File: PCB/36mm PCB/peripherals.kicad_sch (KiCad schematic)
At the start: 21 parts, among them IC2 BMM350, IC6 AS5510-DWLM, J1 Conn_01x04_Pin, U1 BMP581

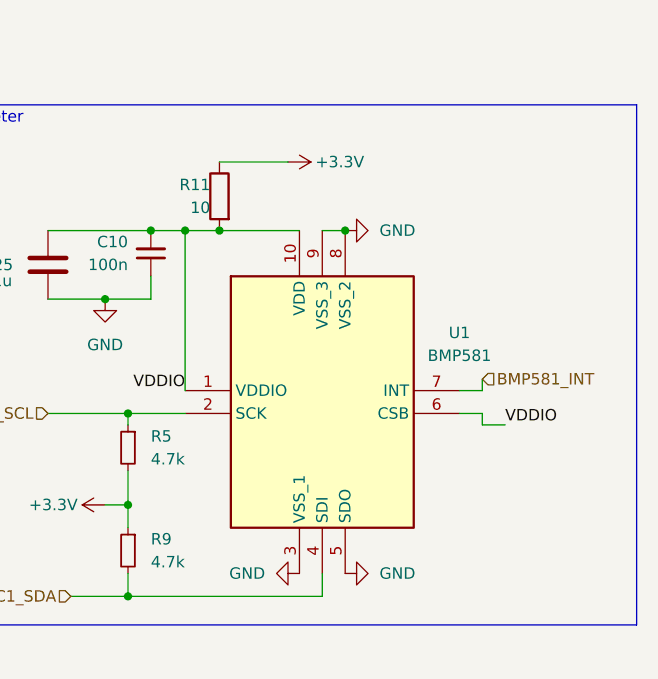
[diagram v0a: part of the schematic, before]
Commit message: Modifs Mathieu
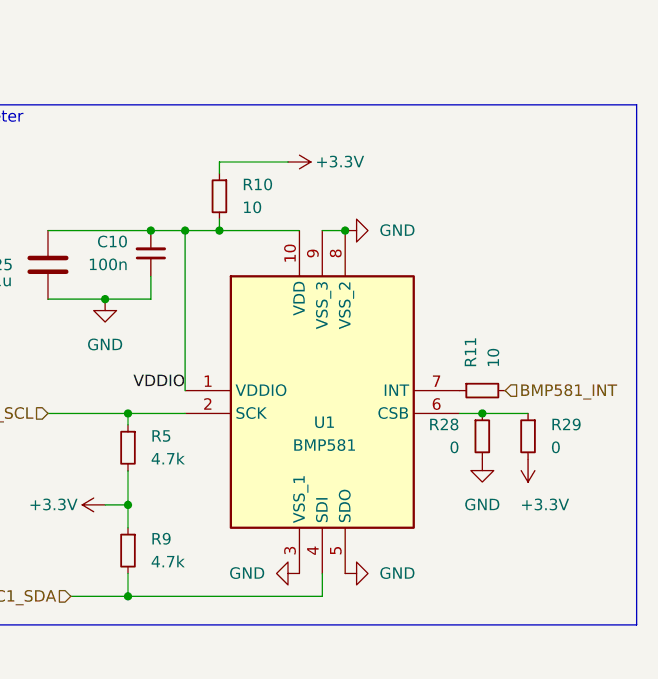
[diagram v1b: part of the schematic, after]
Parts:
- removed R11: 10, Resistor_SMD:R_0402_1005Metric, symbol Device:R
- added R10, R11: 10, Resistor_SMD:R_0201_0603Metric, symbol Device:R_Small
- added R28, R29: 0, Resistor_SMD:R_0201_0603Metric, symbol Device:R_Small
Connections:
- net +3.3V: now also R10.1, R29.2
- net BMP581_INT: now also R11.2; no longer U1.7 (INT)
- net GND: now also R28.2
- net VDDIO: now also R10.2; no longer U1.6 (CSB)
- new net: R11.1, U1.7 (INT)
- new net: R28.1, R29.1, U1.6 (CSB)
